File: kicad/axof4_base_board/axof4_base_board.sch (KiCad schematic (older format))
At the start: 3 parts

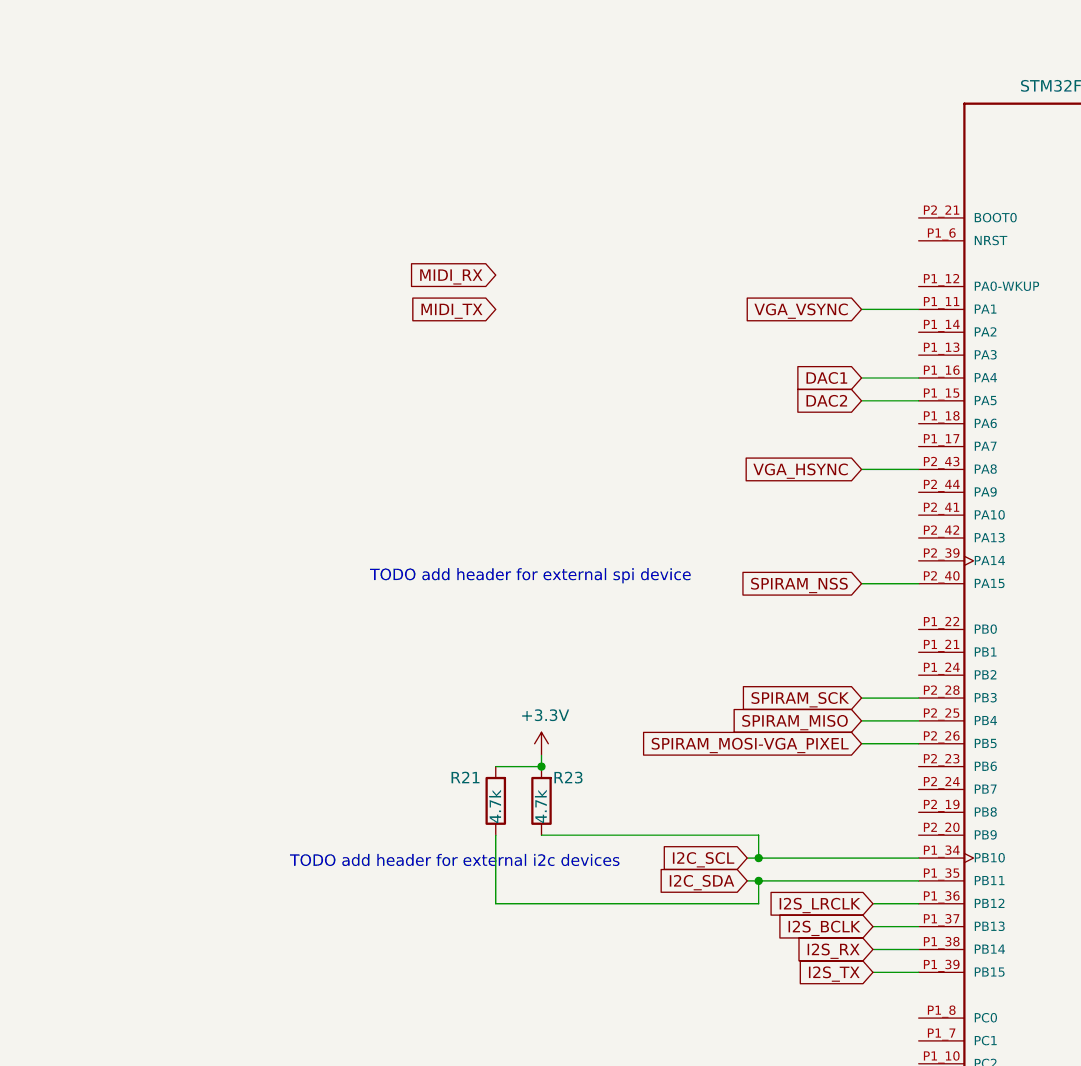
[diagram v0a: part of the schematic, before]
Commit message: kicad pcb backup, hohum axoctrl study
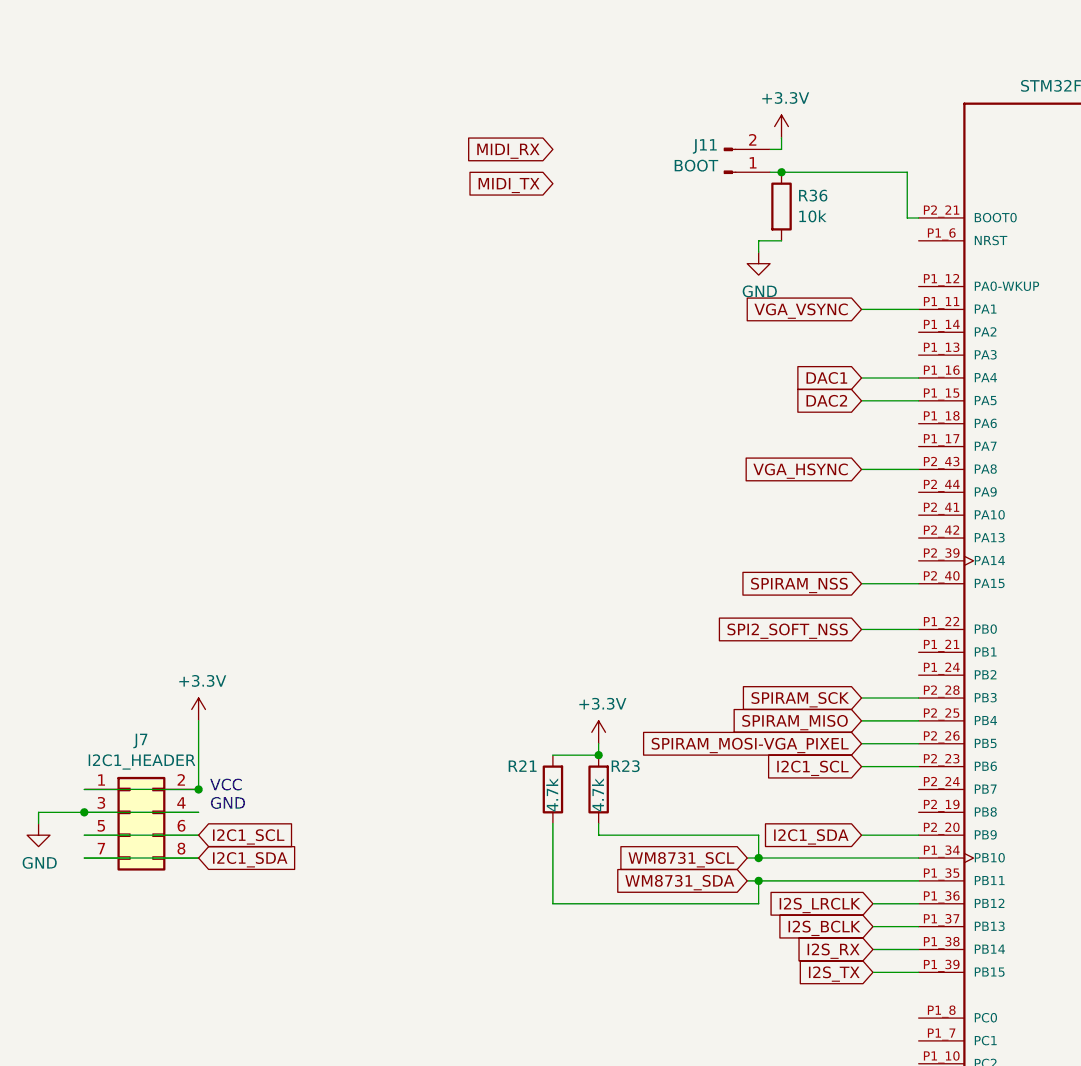
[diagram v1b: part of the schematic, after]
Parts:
- added J11: BOOT, symbol Connector:Conn_01x02_Male
- added J7: I2C1_HEADER, symbol Connector_Generic:Conn_02x04_Odd_Even
- added R36: 10k, symbol Device:R
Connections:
- net +3V3: now also J11.2 (Pin_2), J7.1 (Pin_1), J7.2 (Pin_2)
- net GND: now also J7.3 (Pin_3), J7.4 (Pin_4), R36.2
- net SPI2_SOFT_NSS: now reaches JB1.P1_22 (PB0)
- net I2C1_SDA: now reaches JB1.P2_20 (PB9)
- net I2C1_SDA: now also J7.7 (Pin_7), J7.8 (Pin_8)
- net at JB1.P2_21 (BOOT0): now also J11.1 (Pin_1), R36.1
- net I2C1_SCL: now reaches JB1.P2_23 (PB6)
- net I2C1_SCL: now also J7.5 (Pin_5), J7.6 (Pin_6)
- net I2C_SCL renamed WM8731_SCL
- net I2C_SDA renamed WM8731_SDA
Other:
- note added: "VCC\nGND"
- note removed: "TODO add header for external i2c devices"
- note removed: "TODO add header for external spi device"
- moved on the sheet: R21, R23
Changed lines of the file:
@@
 Wire Wire Line
 	4550 5750 4750 5750
-Text Notes 2000 4500 0    50   ~ 0
-TODO add header for external i2c devices
 Text GLabel 4000 4450 0    50   Input ~ 0
-I2C_SCL
+WM8731_SCL
 Text GLabel 4000 4550 0    50   Input ~ 0
-I2C_SDA
+WM8731_SDA
 Text GLabel 4550 4650 0    50   Input ~ 0
 I2S_LRCLK
@@
 Wire Wire Line
 	4500 3250 4750 3250
-Text Notes 2350 3250 0    50   ~ 0
-TODO add header for external spi device
 Text GLabel 4500 3750 0    50   Input ~ 0
 SPIRAM_SCK
@@
 L axof4_base_board-rescue:R-Device R23
 U 1 1 5EDF8C2D
-P 3100 4200
+P 3350 4150
 AR Path="/5EDF8C2D" Ref="R23"  Part="1"
 AR Path="/5EFC127A/5EDF8C2D" Ref="R?"  Part="1"
-F 0 "R23" H 3050 4100 50  0000 R CNN
-F 1 "4.7k" V 3100 4300 50  0000 R CNN
-F 2 "Resistor_SMD:R_1206_3216Metric_Pad1.42x1.75mm_HandSolder" V 3030 4200 50  0001 C CNN
-F 3 "~" H 3100 4200 50  0001 C CNN
-	1    3100 4200
+F 0 "R23" H 3300 4050 50  0000 R CNN
+F 1 "4.7k" V 3350 4250 50  0000 R CNN
+F 2 "Resistor_SMD:R_1206_3216Metric_Pad1.42x1.75mm_HandSolder" V 3280 4150 50  0001 C CNN
+F 3 "~" H 3350 4150 50  0001 C CNN
+	1    3350 4150
 	-1   0    0    1
 $EndComp
@@
 L axof4_base_board-rescue:+3.3V-power #PWR021
 U 1 1 5EDF8C33
-P 3100 4000
+P 3350 3950
 AR Path="/5EDF8C33" Ref="#PWR021"  Part="1"
 AR Path="/5EFC127A/5EDF8C33" Ref="#PWR?"  Part="1"
-F 0 "#PWR021" H 3100 3850 50  0001 C CNN
-F 1 "+3.3V" H 3115 4173 50  0000 C CNN
-F 2 "" H 3100 4000 50  0001 C CNN
-F 3 "" H 3100 4000 50  0001 C CNN
-	1    3100 4000
-	1    0    0    -1
-$EndComp
-Wire Wire Line
-	3100 4000 3100 4050
-Connection ~ 3100 4050
-Wire Wire Line
-	2900 4050 3100 4050
+F 0 "#PWR021" H 3350 3800 50  0001 C CNN
+F 1 "+3.3V" H 3365 4123 50  0000 C CNN
+F 2 "" H 3350 3950 50  0001 C CNN
+F 3 "" H 3350 3950 50  0001 C CNN
+	1    3350 3950
+	1    0    0    -1
+$EndComp
+Wire Wire Line
+	3350 3950 3350 4000
+Connection ~ 3350 4000
 $Comp
 L axof4_base_board-rescue:R-Device R21
 U 1 1 5EDF8C3C
-P 2900 4200
+P 3150 4150
 AR Path="/5EDF8C3C" Ref="R21"  Part="1"
 AR Path="/5EFC127A/5EDF8C3C" Ref="R?"  Part="1"
-F 0 "R21" H 3100 4100 50  0000 R CNN
-F 1 "4.7k" V 2900 4300 50  0000 R CNN
-F 2 "Resistor_SMD:R_1206_3216Metric_Pad1.42x1.75mm_HandSolder" V 2830 4200 50  0001 C CNN
-F 3 "~" H 2900 4200 50  0001 C CNN
-	1    2900 4200
+F 0 "R21" H 3350 4050 50  0000 R CNN
+F 1 "4.7k" V 3150 4250 50  0000 R CNN
+F 2 "Resistor_SMD:R_1206_3216Metric_Pad1.42x1.75mm_HandSolder" V 3080 4150 50  0001 C CNN
+F 3 "~" H 3150 4150 50  0001 C CNN
+	1    3150 4150
 	-1   0    0    1
 $EndComp
-Wire Wire Line
-	3100 4350 4050 4350
 Wire Wire Line
 	4050 4350 4050 4450
@@
 Wire Wire Line
 	4050 4450 4000 4450
-Wire Wire Line
-	2900 4350 2900 4650
-Wire Wire Line
-	2900 4650 4050 4650
 Wire Wire Line
 	4050 4650 4050 4550
@@
 F1 "midi.sch" 50
 $EndSheet
-Text GLabel 2900 1900 0    50   Input ~ 0
+Text GLabel 3150 1350 0    50   Input ~ 0
 MIDI_RX
-Text GLabel 2900 2050 0    50   Input ~ 0
+Text GLabel 3150 1500 0    50   Input ~ 0
 MIDI_TX
 $Sheet
@@
 F1 "usb.sch" 50
 $EndSheet
+$Comp
+L Connector_Generic:Conn_02x04_Odd_Even J7
+U 1 1 602901E8
+P 1300 4250
+F 0 "J7" H 1350 4567 50  0000 C CNN
+F 1 "I2C1_HEADER" H 1350 4476 50  0000 C CNN
+F 2 "" H 1300 4250 50  0001 C CNN
+F 3 "~" H 1300 4250 50  0001 C CNN
+	1    1300 4250
+	1    0    0    -1
+$EndComp
+Wire Wire Line
+	1600 4150 1100 4150
+Connection ~ 1600 4150
+$Comp
+L power:GND #PWR040
+U 1 1 602A0F05
+P 900 4300
+F 0 "#PWR040" H 900 4050 50  0001 C CNN
+F 1 "GND" H 905 4127 50  0000 C CNN
+F 2 "" H 900 4300 50  0001 C CNN
+F 3 "" H 900 4300 50  0001 C CNN
+	1    900  4300
+	1    0    0    -1
+$EndComp
+Wire Wire Line
+	900  4300 900  4250
+Wire Wire Line
+	900  4250 1100 4250
+Wire Wire Line
+	1100 4450 1600 4450
+Wire Wire Line
+	3150 4300 3150 4650
+Wire Wire Line
+	3350 4350 3350 4300
+Wire Wire Line
+	1600 4350 1100 4350
+Wire Wire Line
+	1600 3850 1600 4150
+Wire Wire Line
+	1100 4250 1600 4250
+Connection ~ 1100 4250
+Text Notes 1650 4250 0    50   ~ 0
+VCC\nGND
+$Comp
+L Connector:Conn_01x02_Male J11
+U 1 1 602C273A
+P 3900 1450
+F 0 "J11" H 3873 1332 50  0000 R CNN
+F 1 "BOOT" H 3873 1423 50  0000 R CNN
+F 2 "" H 3900 1450 50  0001 C CNN
+F 3 "~" H 3900 1450 50  0001 C CNN
+	1    3900 1450
+	1    0    0    1
+$EndComp
+Wire Wire Line
+	4100 1450 4150 1450
+Wire Wire Line
+	4700 1450 4700 1650
+Wire Wire Line
+	4700 1650 4750 1650
+$Comp
+L axof4_base_board-rescue:+3.3V-power #PWR048
+U 1 1 602C979F
+P 4150 1300
+AR Path="/602C979F" Ref="#PWR048"  Part="1"
+AR Path="/5EFC127A/602C979F" Ref="#PWR?"  Part="1"
+F 0 "#PWR048" H 4150 1150 50  0001 C CNN
+F 1 "+3.3V" H 4165 1473 50  0000 C CNN
+F 2 "" H 4150 1300 50  0001 C CNN
+F 3 "" H 4150 1300 50  0001 C CNN
+	1    4150 1300
+	1    0    0    -1
+$EndComp
+Wire Wire Line
+	4150 1300 4150 1350
+Wire Wire Line
+	4150 1350 4100 1350
+$Comp
+L Device:R R36
+U 1 1 602CD2A4
+P 4150 1600
+F 0 "R36" H 4220 1646 50  0000 L CNN
+F 1 "10k" H 4220 1555 50  0000 L CNN
+F 2 "" V 4080 1600 50  0001 C CNN
+F 3 "~" H 4150 1600 50  0001 C CNN
+	1    4150 1600
+	1    0    0    -1
+$EndComp
+Connection ~ 4150 1450
+Wire Wire Line
+	4150 1450 4700 1450
+$Comp
+L power:GND #PWR047
+U 1 1 602CE2E4
+P 4050 1800
+F 0 "#PWR047" H 4050 1550 50  0001 C CNN
+F 1 "GND" H 4055 1627 50  0000 C CNN
+F 2 "" H 4050 1800 50  0001 C CNN
+F 3 "" H 4050 1800 50  0001 C CNN
+	1    4050 1800
+	1    0    0    -1
+$EndComp
+Wire Wire Line
+	4050 1800 4050 1750
+Wire Wire Line
+	4050 1750 4150 1750
+Text GLabel 1600 4350 2    50   Input ~ 0
+I2C1_SCL
+Text GLabel 1600 4450 2    50   Input ~ 0
+I2C1_SDA
+Wire Wire Line
+	3150 4000 3350 4000
+Wire Wire Line
+	3350 4350 4050 4350
+Wire Wire Line
+	3150 4650 4050 4650
+Text GLabel 4500 4050 0    50   Input ~ 0
+I2C1_SCL
+Text GLabel 4500 4350 0    50   Input ~ 0
+I2C1_SDA
+Wire Wire Line
+	4500 4350 4750 4350
+Wire Wire Line
+	4500 4050 4750 4050
+Text GLabel 4500 3450 0    50   Input ~ 0
+SPI2_SOFT_NSS
+Wire Wire Line
+	4500 3450 4750 3450
+$Comp
+L axof4_base_board-rescue:+3.3V-power #PWR041
+U 1 1 603DAAD6
+P 1600 3850
+AR Path="/603DAAD6" Ref="#PWR041"  Part="1"
+AR Path="/5EFC127A/603DAAD6" Ref="#PWR?"  Part="1"
+F 0 "#PWR041" H 1600 3700 50  0001 C CNN
+F 1 "+3.3V" H 1615 4023 50  0000 C CNN
+F 2 "" H 1600 3850 50  0001 C CNN
+F 3 "" H 1600 3850 50  0001 C CNN
+	1    1600 3850
+	1    0    0    -1
+$EndComp
 $EndSCHEMATC
